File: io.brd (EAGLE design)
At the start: 23 x 40 mm, 34 parts, among them J1 SJ-3502-SMT-TR, Q1 2SCR574D3TL1, Q2 2SCR574D3TL1, U1 MCP1703T-5002E, U3 LM386M-1, X1 Antenna

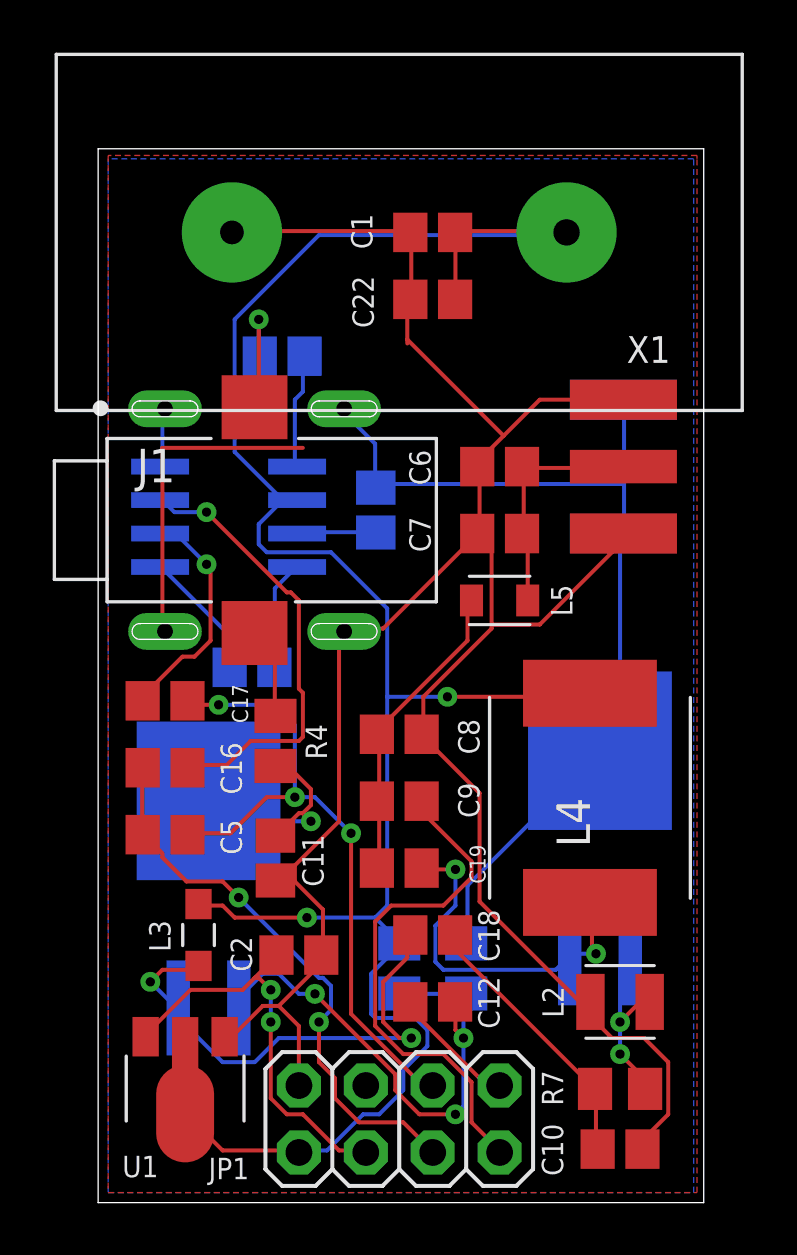
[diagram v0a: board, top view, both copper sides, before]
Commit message: updating layouts and parts
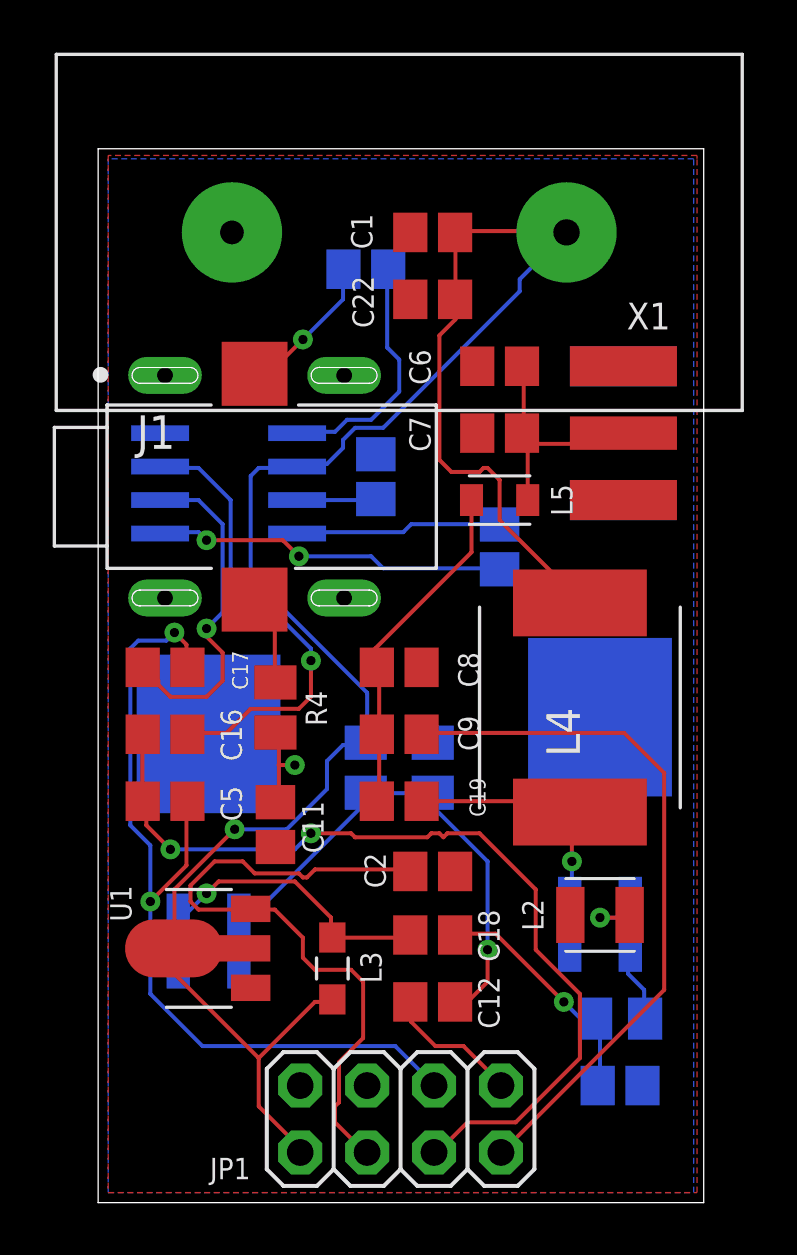
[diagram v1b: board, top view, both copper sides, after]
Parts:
- moved C25 10.5 mm to (15.2, 24.9), turned to 270 degrees
- moved R5 7.73 mm to (12.7, 16.5)
- moved R6 7.73 mm to (10.2, 16.5)
- moved C2 5.99 mm to (12.7, 12.6)
- moved U1 5.36 mm to (3.81, 9.65), turned to 90 degrees
- moved L3 5.24 mm to (8.89, 8.89), turned to 270 degrees
- moved C24 4.58 mm to (10.2, 35.4)
- moved C7 3.81 mm to (15.2, 29.2)
- moved L5 3.81 mm to (15.2, 26.7)
- moved C6 3.81 mm to (15.2, 31.8)
- moved L4 3.45 mm to (18.3, 18.8)
- moved L2 3.39 mm to (19.1, 10.9)
- moved R7 2.67 mm to (19.8, 6.99), flipped to the bottom, turned to 180 degrees
- moved C19 2.54 mm to (11.4, 15.2)
- moved C9 2.54 mm to (11.4, 17.8)
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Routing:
- net GND: track 142.9 -> 0.00 mm
- net OUT_A: track 21.4 -> 34.3 mm
- net 6V_DC: track 15.7 -> 25.6 mm, vias 2 -> 0
- net N$13: track 4.92 -> 13.5 mm, vias 0 -> 2
- net OUT_B: track 25.7 -> 33.5 mm, vias 3 -> 2
- net N$21: track 19.0 -> 11.5 mm, vias 2 -> 1
- net ANT_IN: track 19.7 -> 26.8 mm
- net VIN: track 83.1 -> 76.1 mm, vias 2 -> 1
- net N$14: track 4.36 -> 9.37 mm
- net N$10: track 9.25 -> 13.0 mm
- net N$12: track 4.18 -> 7.84 mm
- net N$24: track 13.6 -> 10.7 mm, vias 2 -> 1
- net N$20: track 8.77 -> 7.24 mm
- net N$25: track 11.9 -> 13.2 mm
- net N$22: track 10.4 -> 9.31 mm, vias 0 -> 1
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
